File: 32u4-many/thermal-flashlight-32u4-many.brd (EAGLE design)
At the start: 49.3 x 46.2 mm, 36 parts, among them IC2 MCP73831, IC3 ATMEGA32U4-AU, IC4 MCP1700-33, J1 AYZ0202, J2 1X2-3.5MM, Q4 BSS123, U1 MLX90614_, X1 USBSMD, X3 8MHz

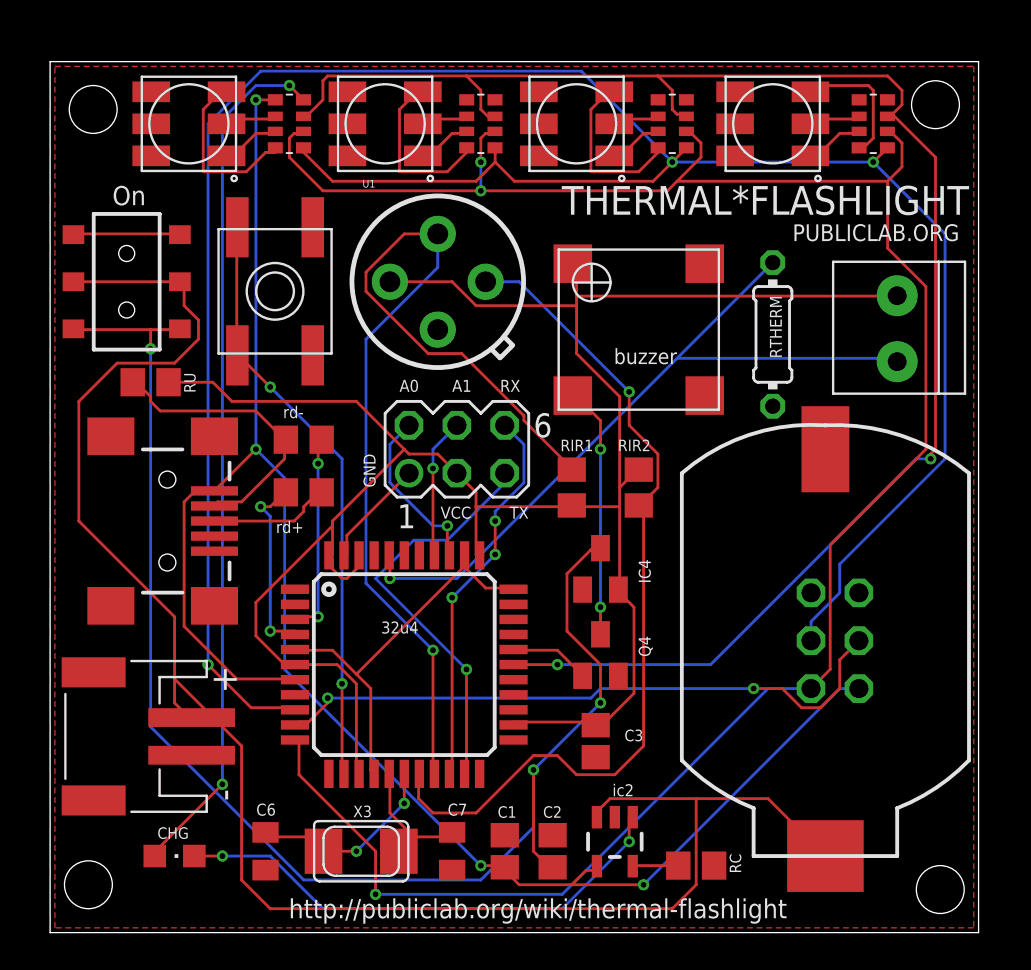
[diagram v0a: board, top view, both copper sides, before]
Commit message: update
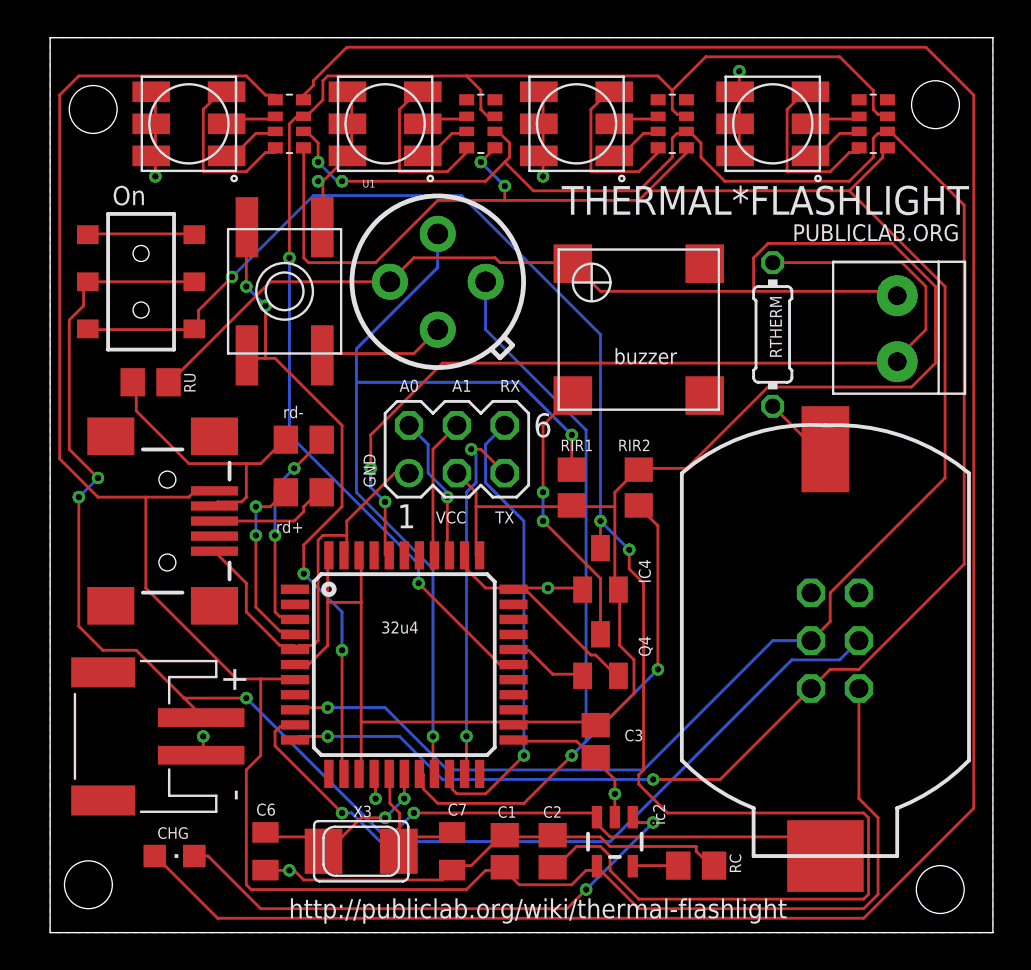
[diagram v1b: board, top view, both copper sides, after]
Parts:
- moved J1 0.76 mm to (5.08, 34.5)
- moved CN1 0.51 mm to (4.57, 10.4)
- moved BTN 0.51 mm to (12.7, 34.0)
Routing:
- net GND: track 27.7 -> 108.3 mm, vias 0 -> 9
- net N$10: track 46.3 -> 123.2 mm, vias 2 -> 0
- net VBUS: track 92.0 -> 114.6 mm, vias 4 -> 0
- net VDD: track 75.6 -> 96.2 mm
- net SCK: track 127.3 -> 106.9 mm
- net VBAT: track 92.2 -> 73.0 mm, vias 0 -> 4
- net VCC: track 119.7 -> 138.4 mm
- net D8: track 87.8 -> 75.5 mm
- net A4: track 40.4 -> 49.8 mm, vias 1 -> 2
- net SCL: track 46.0 -> 52.4 mm, vias 1 -> 2
- net MISO: track 113.4 -> 107.5 mm, vias 3 -> 4
- net MOSI: track 33.7 -> 39.5 mm, vias 2 -> 1
- net SDA: track 52.4 -> 46.6 mm, vias 1 -> 2
- net D0/RX: track 20.5 -> 24.5 mm, vias 3 -> 1
- net RST: track 31.4 -> 34.2 mm, vias 2 -> 4
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- added copper zone on layer 16, net GND
- removed copper zone on layer 1, net GND
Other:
- board size 49.3 x 46.2 mm -> 50 x 47.5 mm
- board text added: "MISO"
- board text added: "MOSI"
- board text added: "RESET"
- board text added: "SCK"
- board text added: "VBUS"
